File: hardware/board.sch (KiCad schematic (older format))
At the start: 41 parts, among them J1 Conn_01x03_Male, J2 Conn_01x03_Male, J3 Conn_01x06, J4 Conn_01x06_Female, J5 Conn_01x06, J8 Conn_01x04, Q1 AO3400A, Q2 AO3400A, SW1 SW_Push, SW2 SW_Push, U1 HT7850-1-SOT89, U2 HT7833-1-SOT89, U3 ESP32-WROOM-32

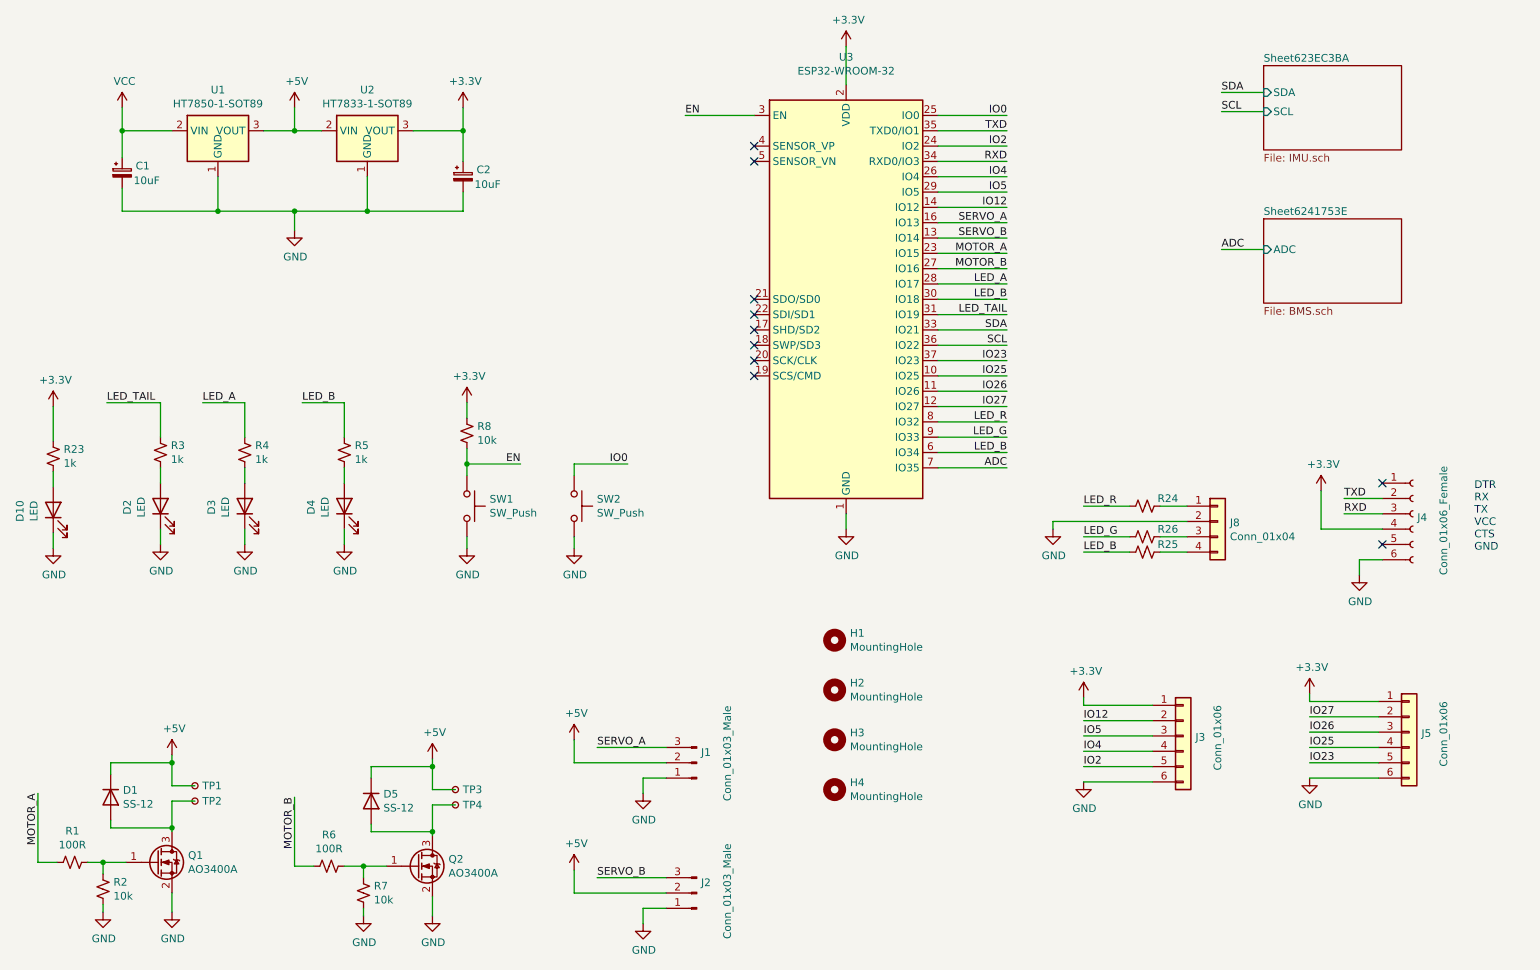
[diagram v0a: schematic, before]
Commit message: PCB: Minor changes
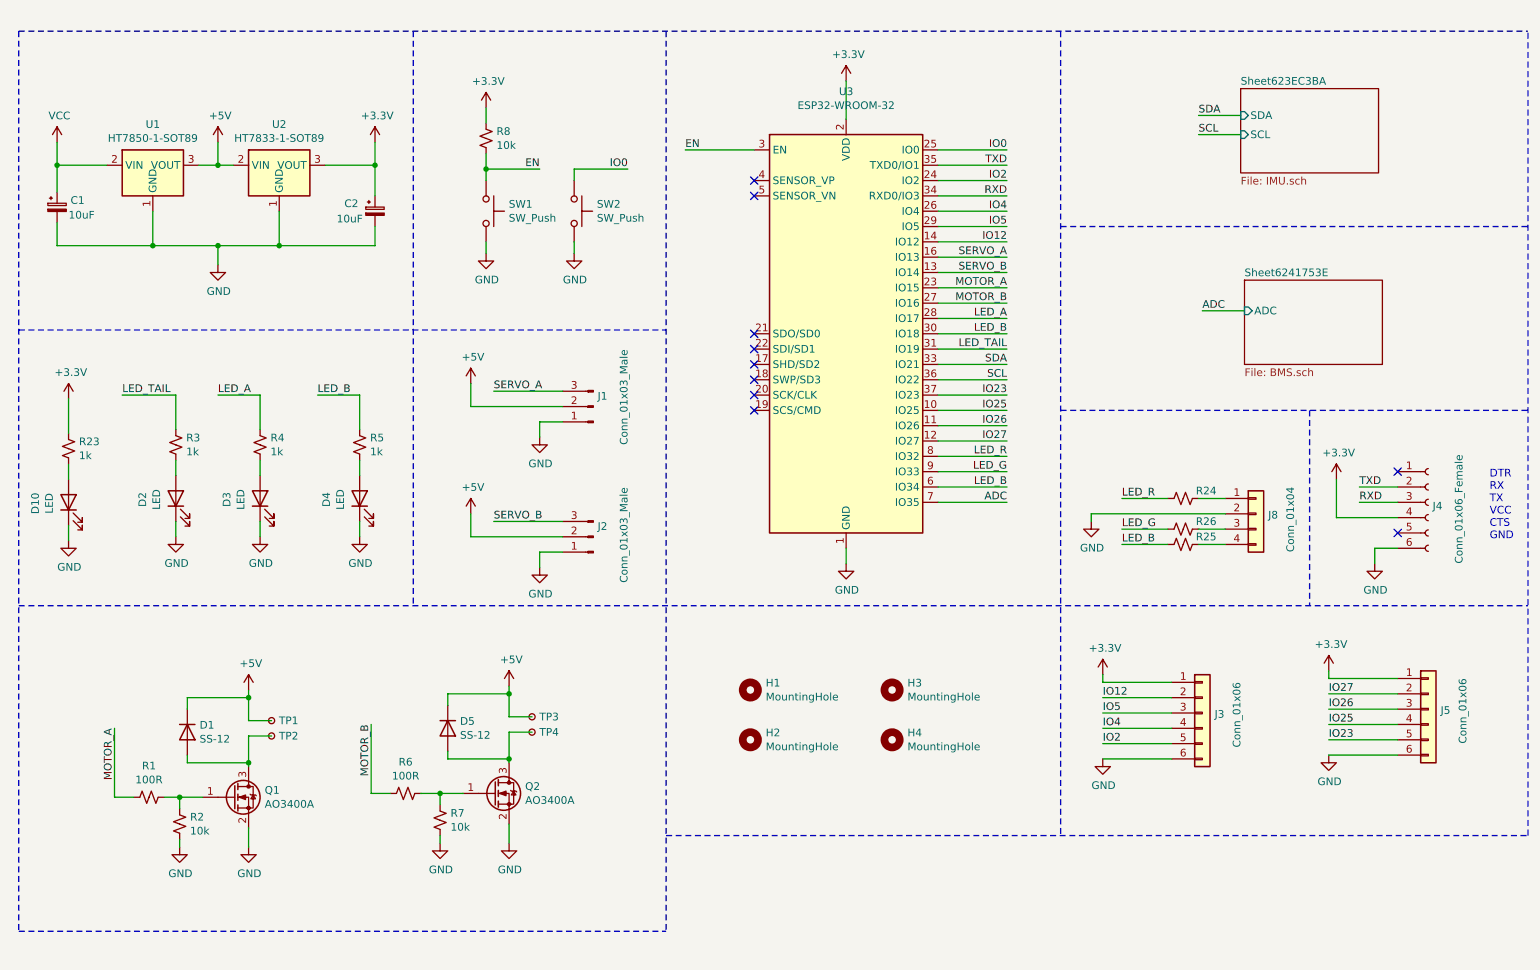
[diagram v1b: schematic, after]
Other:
- moved on the sheet: C1, C2, D1, D10, D2, D3, D4, D5, H1, H2, H3, H4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
